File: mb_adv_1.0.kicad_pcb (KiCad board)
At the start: 2 copper layers, 50 x 54 mm, 10 parts, among them M2 MountingHole_2.1mm, SW2 SW_SP3T, U2 gba_link_cable, U3 BOB-12009

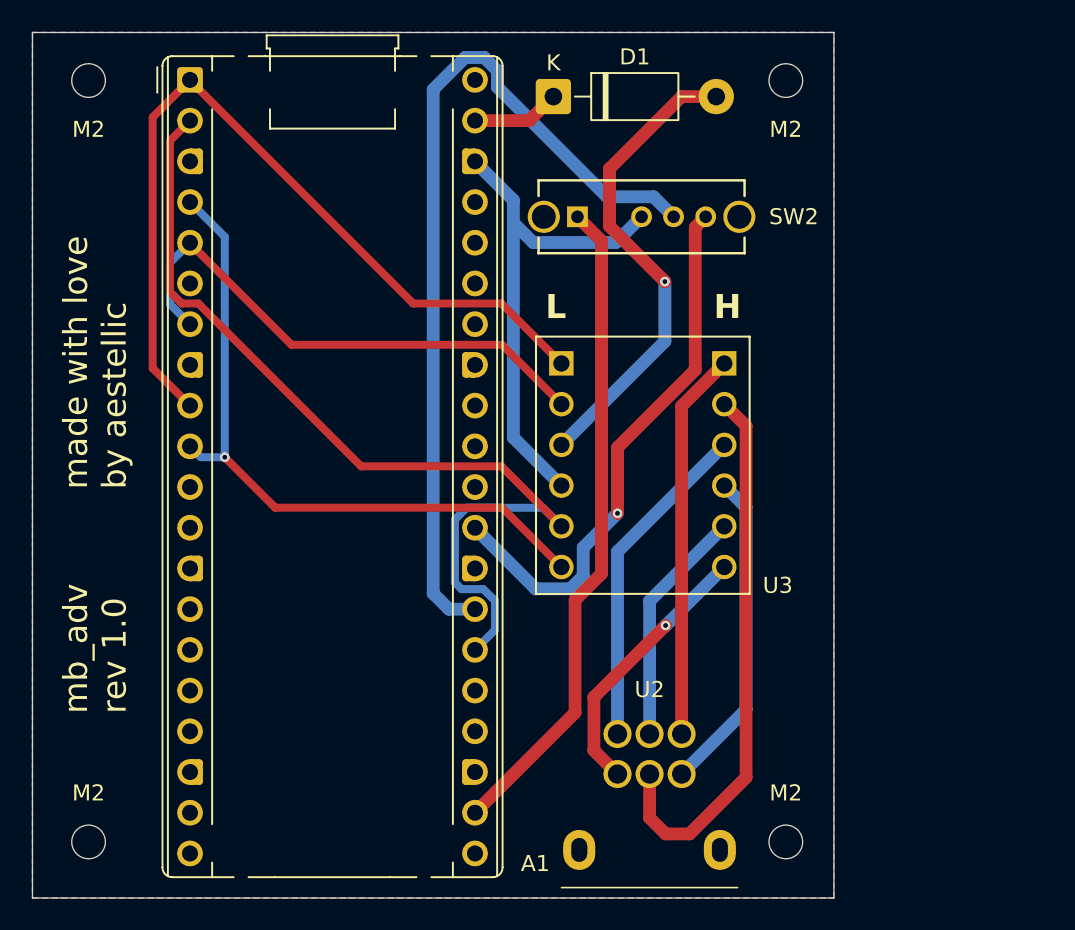
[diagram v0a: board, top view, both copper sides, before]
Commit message: add microSD card
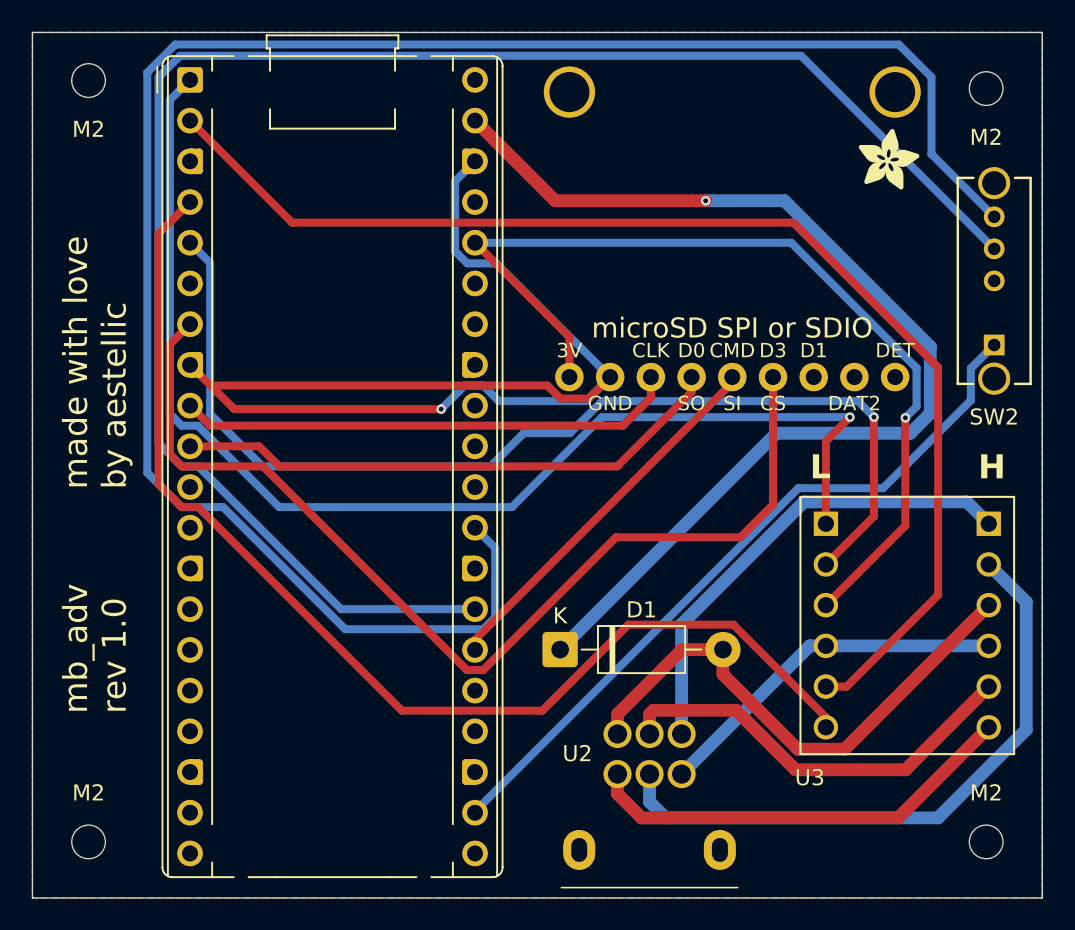
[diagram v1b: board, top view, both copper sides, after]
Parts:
- added U1: Adafruit-MicroSD-SPI-4682, adafruit:adafruit_4682, F.Cu at (161.9, 90.3)
- moved D1 34.5 mm to (150.9, 116.5)
- moved SW2 27.2 mm to (178.0, 97.5), turned to 180 degrees
- moved U3 19.3 mm to (172.6, 115.0)
- moved M2 12.5 mm to (177.5, 81.5)
- moved M2 12.5 mm to (177.5, 128.5)
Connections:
- A1 pad 10: PSO -> uSO
- A1 pad 26: PSI -> uSI
- A1 pad 36: unconnected-(A1-3V3-Pad36) -> LV
- A1 pad 7: PSD -> uSD
- A1 pad 9: PSC -> uSC
- D1 pad 2: LV -> HV
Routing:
- net OPT_3: track 34.3 -> 118.0 mm, vias 1 -> 0
- net uSD: track 0.00 -> 64.1 mm
- net Net-(A1-VSYS): track 4.74 -> 67.6 mm, vias 0 -> 1
- net OPT_2: track 55.0 -> 104.5 mm
- net GND: track 52.1 -> 97.0 mm, vias 0 -> 1
- net uSO: track 0.00 -> 34.7 mm
- net PSD: track 33.5 -> 66.5 mm, vias 0 -> 1
- net uSC: track 0.00 -> 31.3 mm
- net LV: track 29.9 -> 58.7 mm
- net PSO: track 43.5 -> 71.1 mm, vias 1 -> 0
- net uSI: track 0.00 -> 23.7 mm
- net PSC: track 52.8 -> 75.8 mm, vias 0 -> 1
- net PSI: track 60.0 -> 76.6 mm
- net HV: track 20.8 -> 33.3 mm
- net Net-(U2-SI): track 14.9 -> 26.2 mm
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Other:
- board size 50 x 54 mm -> 63 x 54 mm

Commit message: finalize PCB
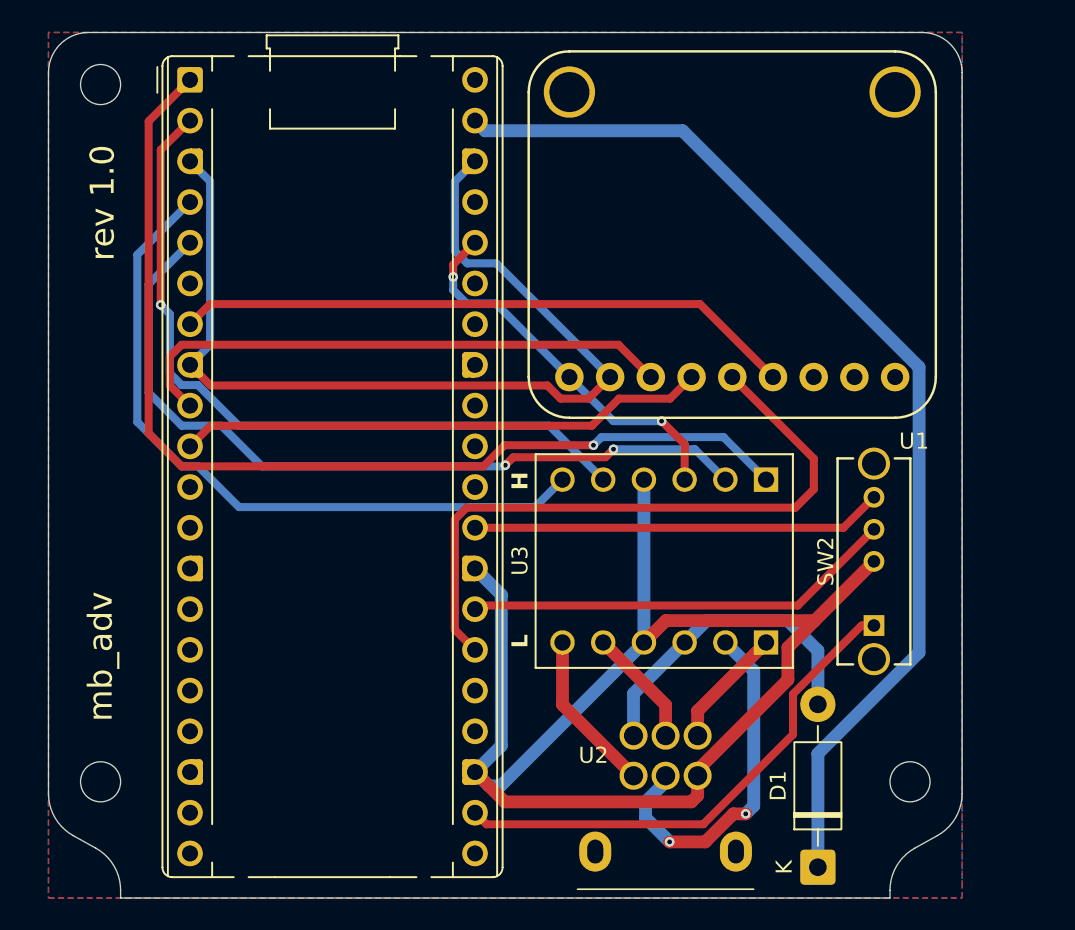
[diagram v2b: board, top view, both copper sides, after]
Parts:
- removed M2 (x4): MountingHole_2.1mm, MountingHole:MountingHole_2.1mm
- added M2.5: MountingHole_2.5mm, MountingHole:MountingHole_2.5mm, F.Cu at (122.2, 81.2)
- added M2.5: MountingHole_2.5mm, MountingHole:MountingHole_2.5mm, F.Cu at (122.2, 124.8)
- added M2.5: MountingHole_2.5mm, MountingHole:MountingHole_2.5mm, F.Cu at (172.8, 124.8)
- moved D1 21.0 mm to (167.0, 130.1), turned to 90 degrees
- moved SW2 19.0 mm to (170.5, 115.0)
- moved U3 15.7 mm to (157.4, 111.0), turned to -90 degrees
- moved U2 1.01 mm to (157.5, 125.4)
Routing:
- net OPT_3: track 118.0 -> 25.7 mm
- net OPT_2: track 104.5 -> 27.0 mm
- net GND: track 97.0 -> 145.1 mm, vias 1 -> 0
- net LV: track 58.7 -> 24.1 mm, vias 1 -> 2
- net PSI: track 76.6 -> 46.5 mm, vias 0 -> 1
- net PSO: track 71.1 -> 44.5 mm
- net uSD: track 64.1 -> 38.8 mm
- net Net-(U2-SC): track 29.7 -> 7.58 mm
- net Net-(U2-SI): track 26.2 -> 7.42 mm
- net uSI: track 23.7 -> 41.3 mm
- net Net-(U2-SO): track 27.4 -> 10.1 mm
- net PSD: track 66.5 -> 49.5 mm, vias 1 -> 2
- net Net-(U2-SD): track 39.2 -> 22.4 mm, vias 0 -> 2
- net OPT_1: track 45.7 -> 31.9 mm
- net HV: track 33.3 -> 20.1 mm
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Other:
- board size 63 x 54 mm -> 57 x 54 mm
- board text added: "Made by aestellic Thank you to: cozydelaney Ashton Herron (Starlark) prof.beans Cilerba Bucket Mouse wheat jerm"
- board text added: "mb_adv"
- board text added: "rev 1.0"
- board text removed: "M2"
- board text removed: "Thank you to: cozydelaney Ashton Herron (Starlark) prof.beans Cilerba Bucket Mouse wheat jerm and you!"
- board text removed: "made with love by aestellic"
- board text removed: "mb_adv rev 1.0"
